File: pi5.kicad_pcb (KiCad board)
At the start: 2 copper layers, 319 parts, among them J1 USB_C_Receptacle_GCT_USB4105-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, J10 RJ45_Wuerth_7499111446_Horizo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, J11 USB_A_Wuerth_61400826021_Hori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, J12 USB3_A_Molex_48406-0001_Horiz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, J13 HDMI_Micro-D_Molex_46765-1xxx, J14 PinHeader_2x02_P2.54mm_Vertic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, J17 JST_SH_BM04B-SRSS-TB_1x04-1MP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, J2 HDMI_Micro-D_Molex_46765-1xxx, J20 52559-1652, J3 F32Q-1A7H1-11022, J4 F32Q-1A7H1-11022, J8 PinHeader_2x20_P2.54mm_Vertic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, J9 104031-0811, U5 DA9091

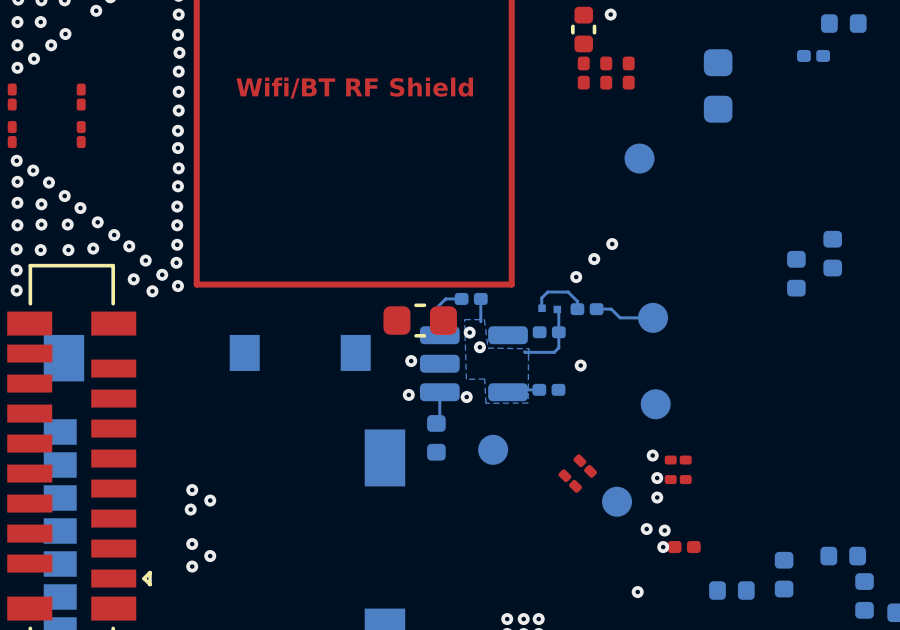
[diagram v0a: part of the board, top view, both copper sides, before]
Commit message: connect sw detect
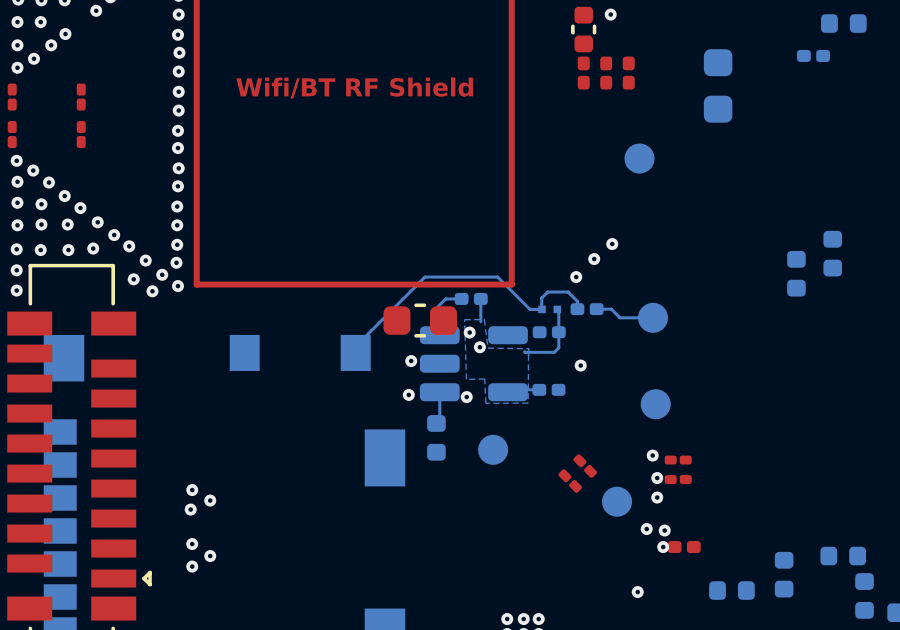
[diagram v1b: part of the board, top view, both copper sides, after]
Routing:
- net SD_SW_DETECT: track 4.04 -> 11.9 mm
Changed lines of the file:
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@@
 	(footprint ""
 		(layer "F.Cu")
-		(at 115.51 86.19)
+		(at 115.51 86.23)
 		(property "Reference" ""
 			(at 0 0 0)
@@
 	)
 	(segment
+		(start 109.3 87.46)
+		(end 109.3 87.680001)
+		(width 0.1)
+		(layer "B.Cu")
+		(net "SD_SW_DETECT")
+	)
+	(segment
 		(start 115.5 85.85)
 		(end 115.5 86.23)
@@
 	)
 	(segment
+		(start 115.11 86.23)
+		(end 114.03 85.15)
+		(width 0.1)
+		(layer "B.Cu")
+		(net "SD_SW_DETECT")
+	)
+	(segment
 		(start 116.38 85.65)
 		(end 115.7 85.65)
@@
 		(width 0.1)
 		(layer "B.Cu")
+		(net "SD_SW_DETECT")
+	)
+	(segment
+		(start 115.51 86.23)
+		(end 115.11 86.23)
+		(width 0.1)
+		(layer "B.Cu")
+		(net "SD_SW_DETECT")
+	)
+	(segment
+		(start 111.61 85.15)
+		(end 109.3 87.46)
+		(width 0.1)
+		(layer "B.Cu")
+		(net "SD_SW_DETECT")
+	)
+	(segment
+		(start 114.03 85.15)
+		(end 111.61 85.15)
+		(width 0.1)
+		(layer "B.Cu")
